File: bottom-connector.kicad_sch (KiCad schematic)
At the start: 12 parts, among them J1 Compute-Module-4_Plug_Connect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, Q3 DZDH0401DW, Q9 AO3401A, U20 NTS0102_XSON, U21 NTS0102_XSON

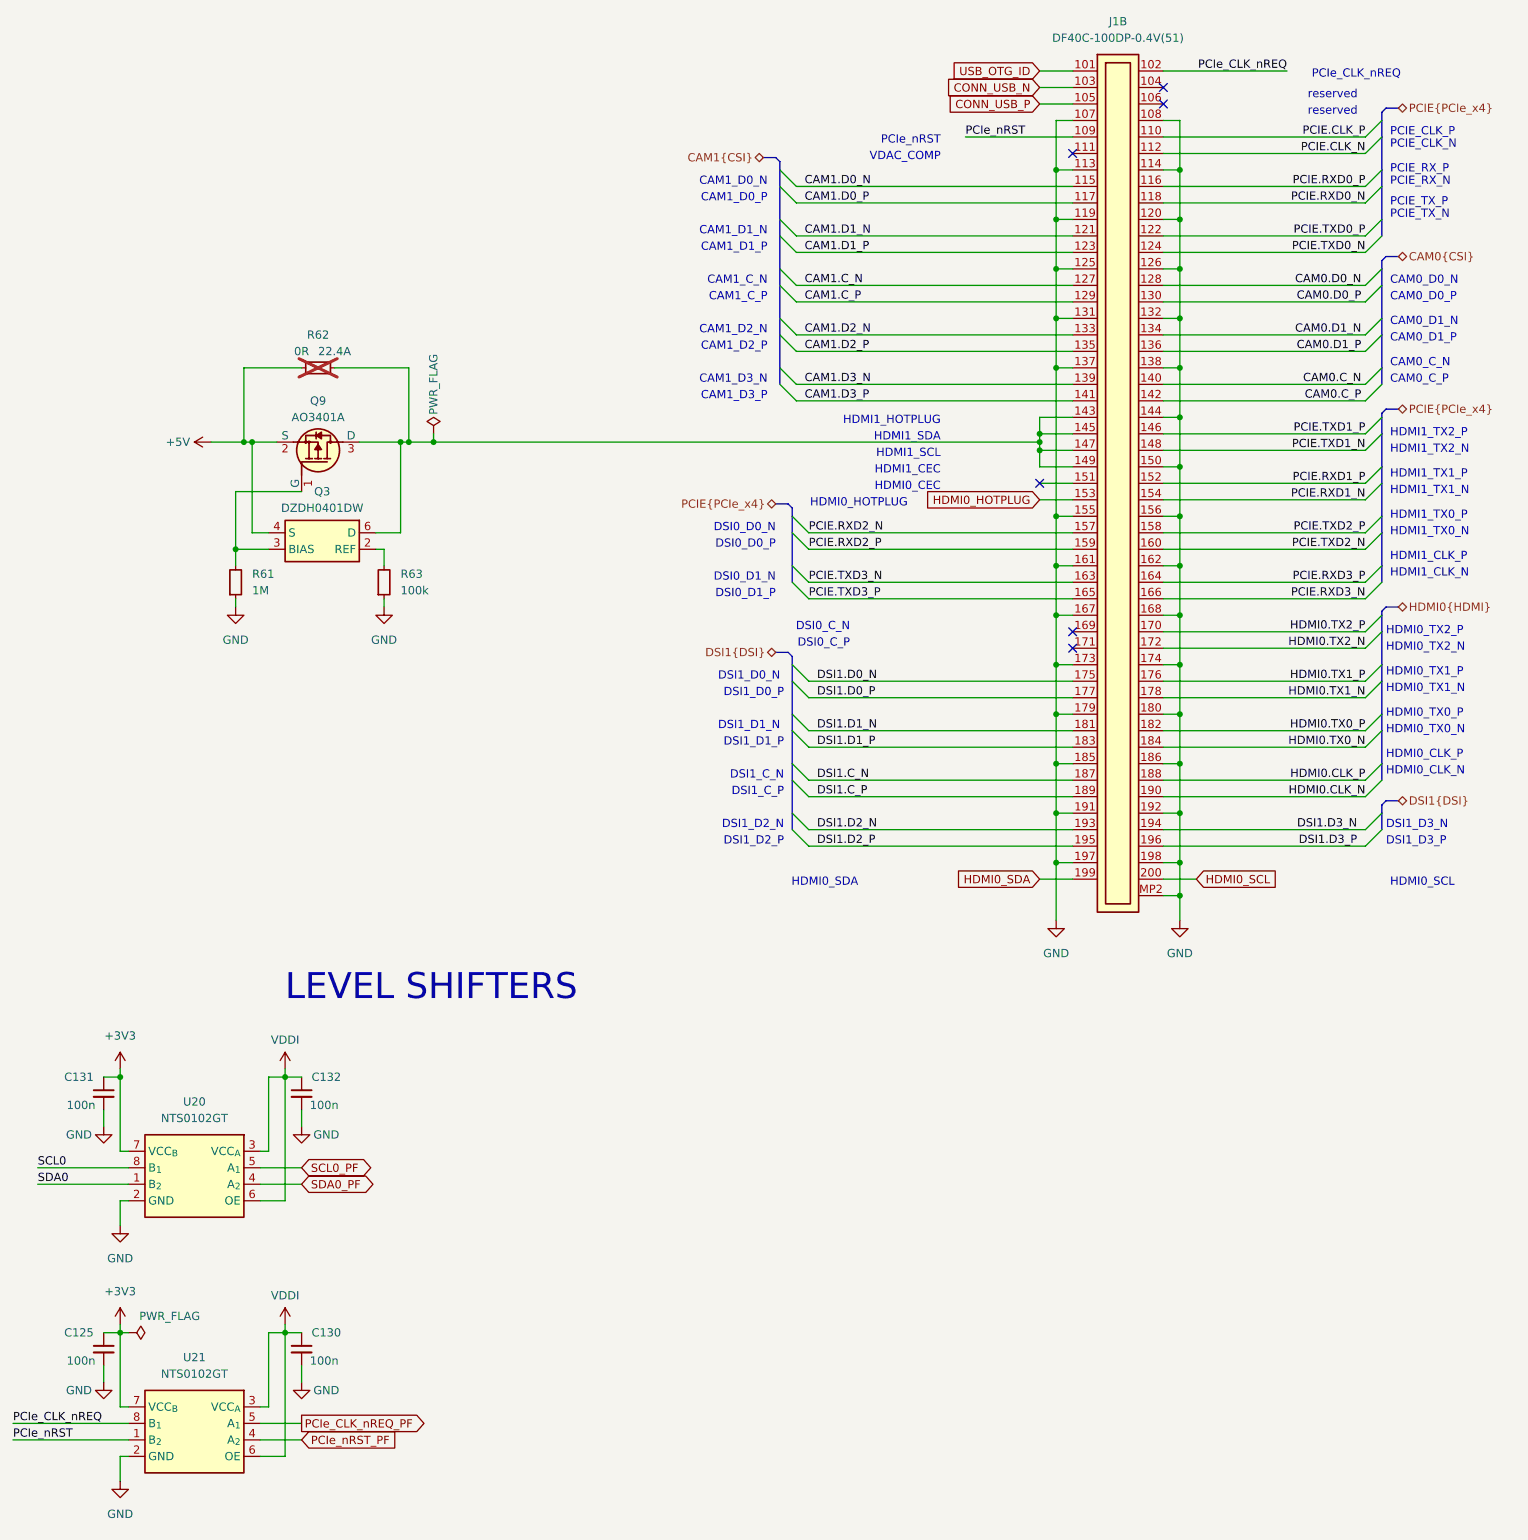
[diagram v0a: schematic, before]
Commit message: [#57505] Finish defining buses
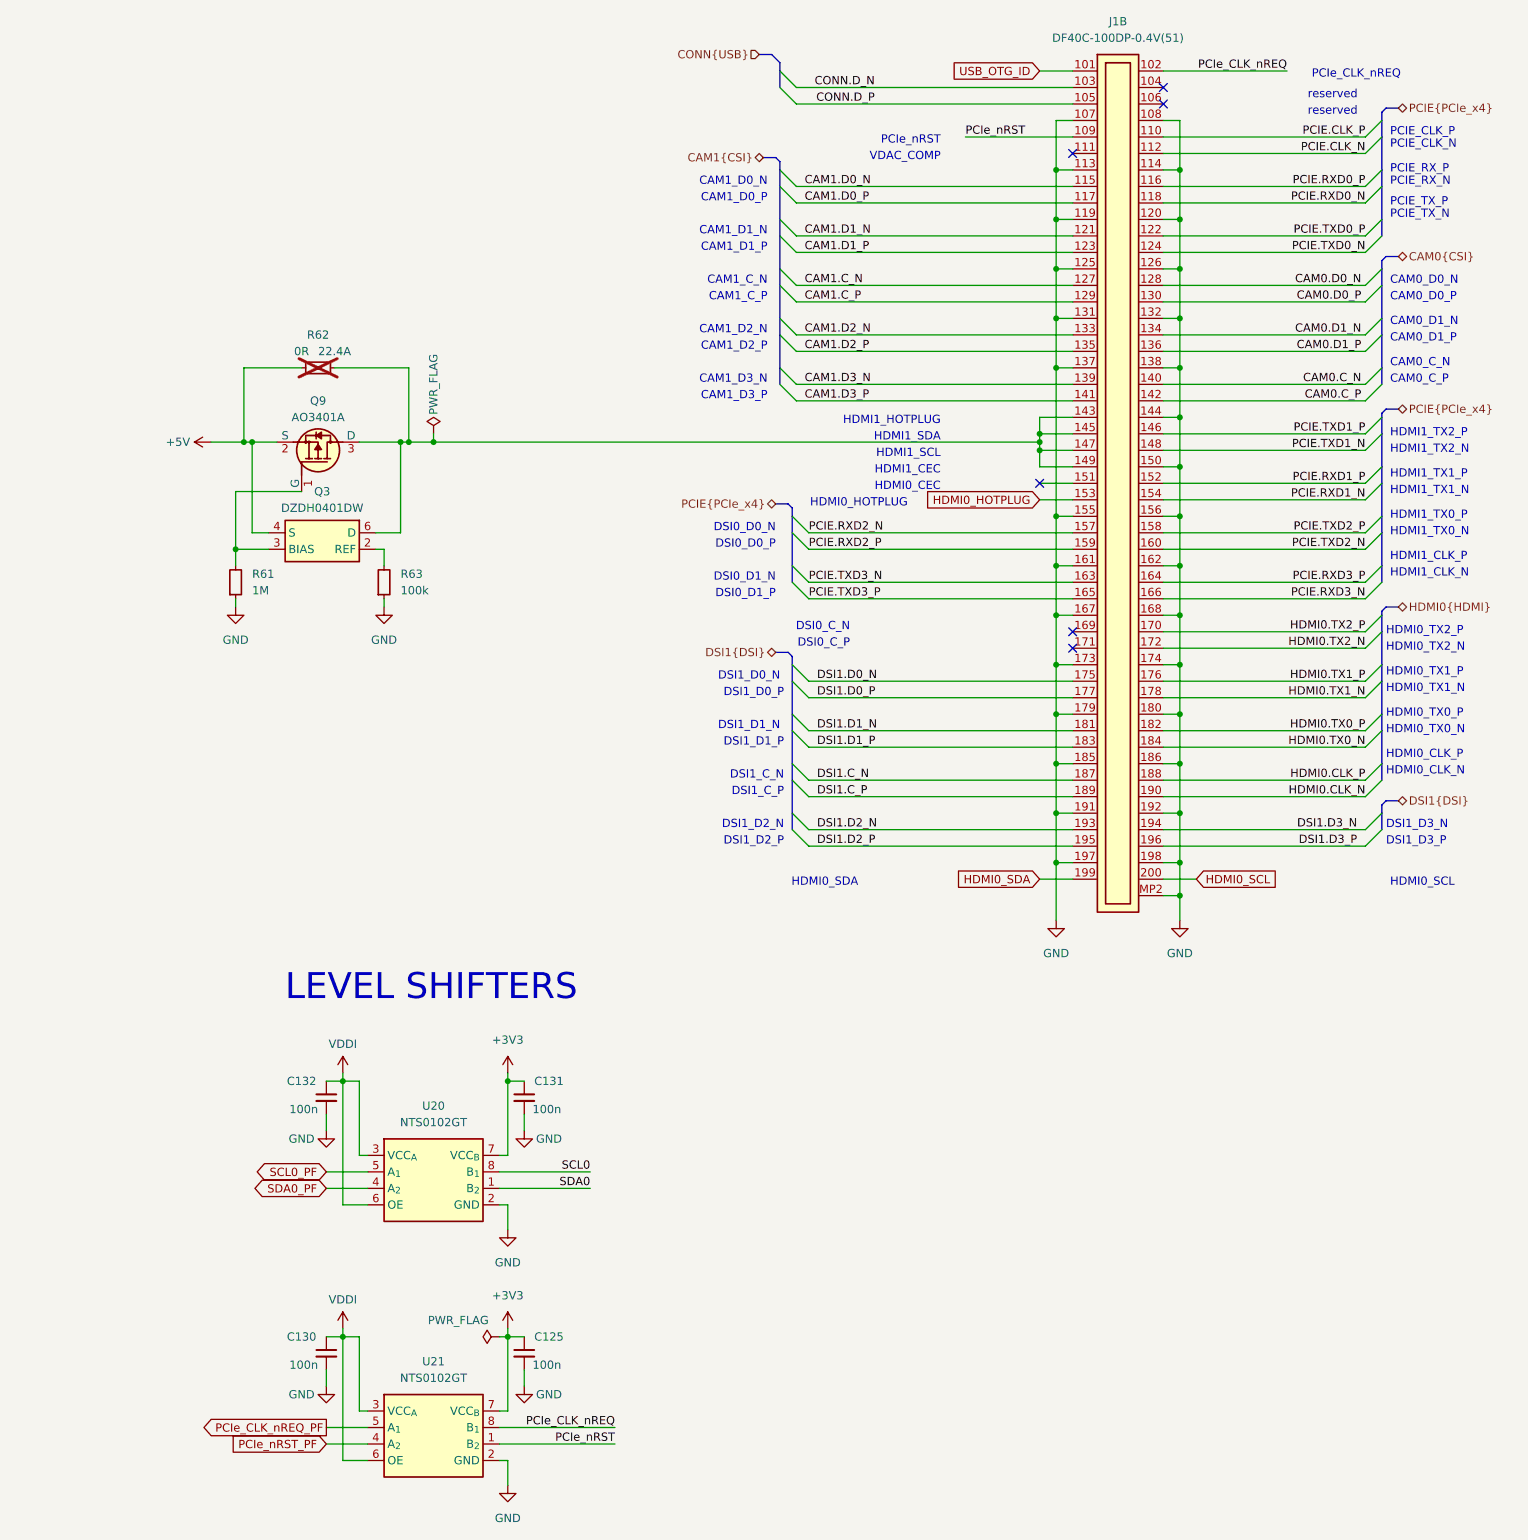
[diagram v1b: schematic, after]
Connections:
- net CONN_USB_N renamed CONN.D_N
- net CONN_USB_P renamed CONN.D_P
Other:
- moved on the sheet: C125, C130, C131, C132, U20, U21
